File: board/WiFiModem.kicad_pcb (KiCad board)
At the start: 2 copper layers, 88.9 x 61 mm, 46 parts, among them J1 DB9_Female, J2 DB25_Female, J3 Barrel_Jack_Switch, J4 PRG, SW1 SW_Push, SW2 SW_Push, U1 ESP-12E, U2 LM7805_TO220, U3 MAX232, U4 LT1117-3.3, U5 MAX232

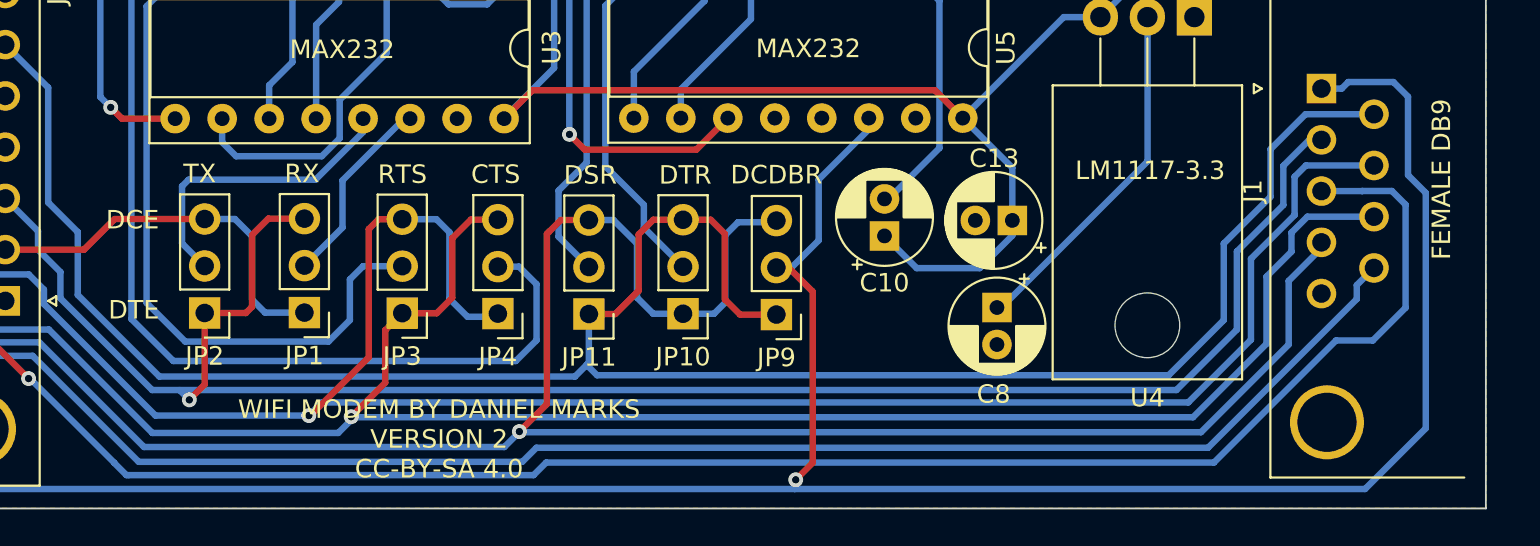
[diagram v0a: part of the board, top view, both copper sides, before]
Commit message: Moved around some traces
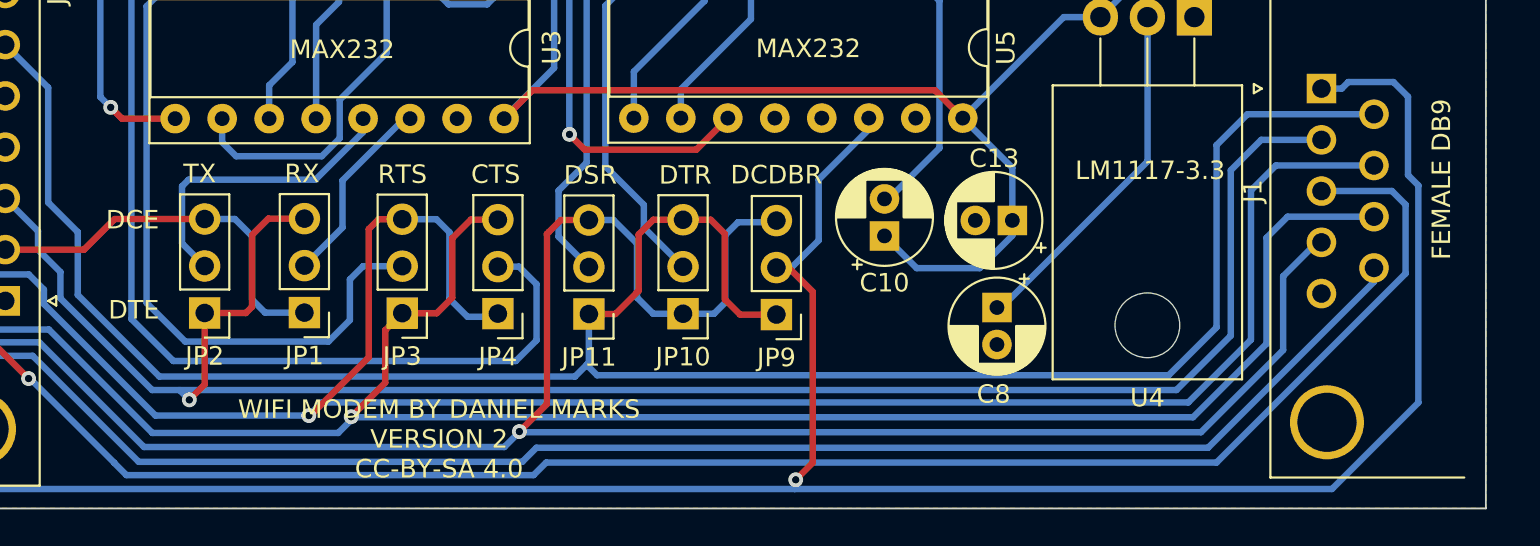
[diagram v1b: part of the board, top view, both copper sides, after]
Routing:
- net DSR: track 118.3 -> 120.2 mm
- net TXD: track 101.7 -> 103.3 mm
- net DCD: track 168.0 -> 166.6 mm
- net RXD: track 120.5 -> 119.4 mm
- net CTS: track 118.5 -> 119.4 mm
- net RTS: track 120.9 -> 121.5 mm
